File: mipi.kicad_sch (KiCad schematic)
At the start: 14 parts, among them J10 Conn_01x30_MountingPin, J9 Conn_01x30_MountingPin

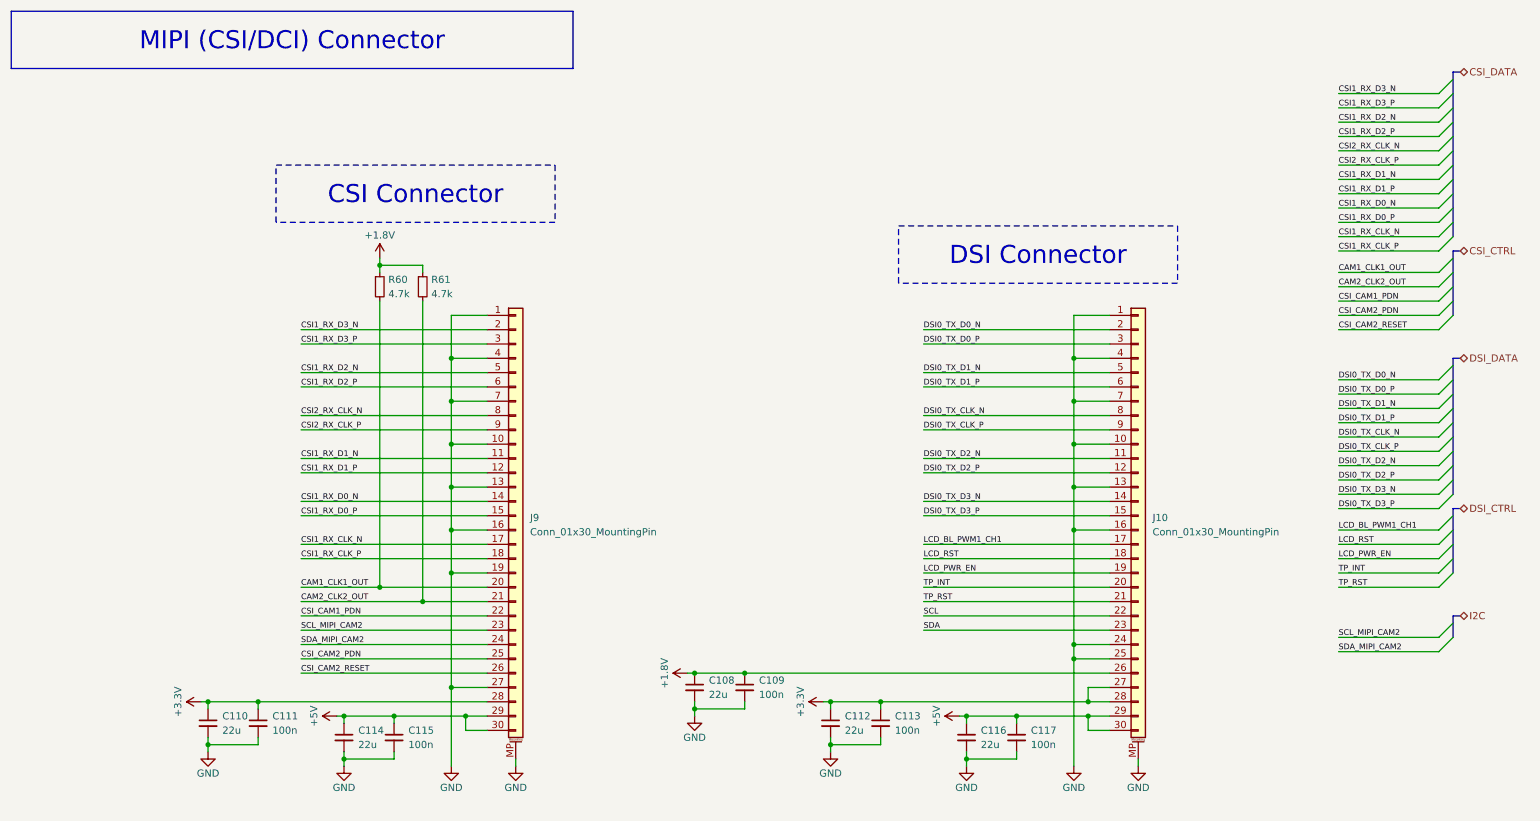
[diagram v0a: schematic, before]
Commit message: Add files via upload
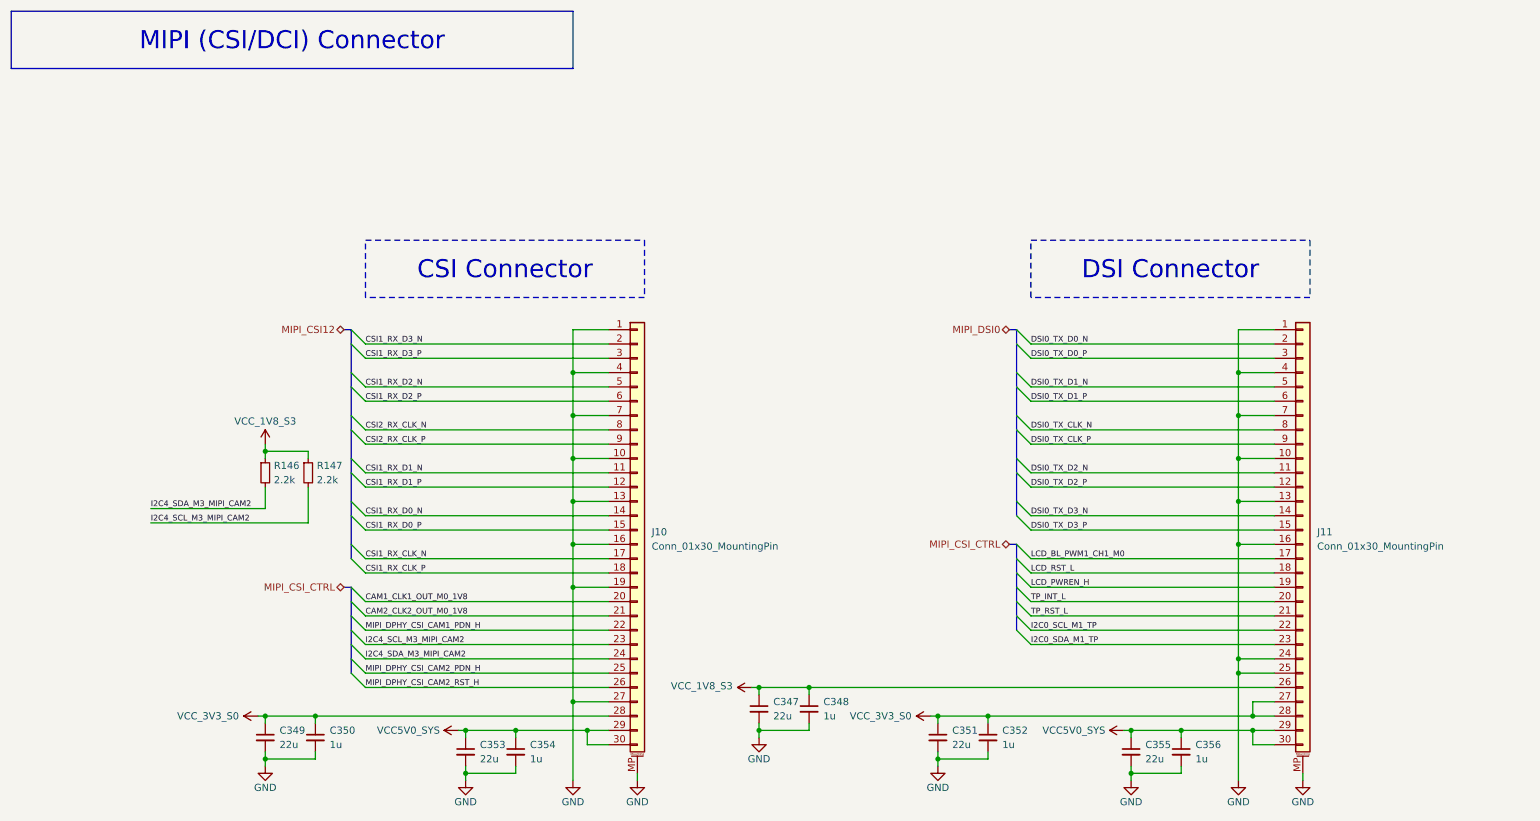
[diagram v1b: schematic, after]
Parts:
- C348: renamed from C109; value 100n -> 1u
- C350: renamed from C111; value 100n -> 1u
- C352: renamed from C113; value 100n -> 1u
- C354: renamed from C115; value 100n -> 1u
- C356: renamed from C117; value 100n -> 1u
- R146: renamed from R60; value 4.7k -> 2.2k
- R147: renamed from R61; value 4.7k -> 2.2k
- renumbered C108 to C347, C110 to C349, C112 to C351, C114 to C353, C116 to C355, J9 to J10, J10 to J11
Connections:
- net +1.8V renamed VCC_1V8_S3
- net +3.3V renamed VCC_3V3_S0
- net +5V renamed VCC5V0_SYS
- net CAM1_CLK1_OUT renamed CAM1_CLK1_OUT_M0_1V8
- net CAM1_CLK1_OUT_M0_1V8: no longer R146.2
- net CAM2_CLK2_OUT renamed CAM2_CLK2_OUT_M0_1V8
- net CAM2_CLK2_OUT_M0_1V8: no longer R147.2
- net CSI_CAM1_PDN renamed MIPI_DPHY_CSI_CAM1_PDN_H
- net CSI_CAM2_PDN renamed MIPI_DPHY_CSI_CAM2_PDN_H
- net CSI_CAM2_RESET renamed MIPI_DPHY_CSI_CAM2_RST_H
- net LCD_BL_PWM1_CH1 renamed LCD_BL_PWM1_CH1_M0
- net LCD_PWR_EN renamed LCD_PWREN_H
- net LCD_RST renamed LCD_RST_L
- net SCL renamed I2C0_SCL_M1_TP
- net SCL_MIPI_CAM2 renamed I2C4_SCL_M3_MIPI_CAM2
- net I2C4_SCL_M3_MIPI_CAM2: now also R147.2
- net SDA renamed I2C0_SDA_M1_TP
- net SDA_MIPI_CAM2 renamed I2C4_SDA_M3_MIPI_CAM2
- net I2C4_SDA_M3_MIPI_CAM2: now also R146.2
- net TP_INT renamed TP_INT_L
- net TP_RST renamed TP_RST_L
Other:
- moved on the sheet: C347, C348, C349, C350, C351, C352, C353, C354, C355, C356, J10, J11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
